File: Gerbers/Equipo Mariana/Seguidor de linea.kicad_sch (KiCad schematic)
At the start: 23 parts, among them J1 VCC, J11 I2C PROTOCOL, J2 MOTOR A, J3 MOTOR B, J4 Regleta_Jabots, J5 TURBIBNA, J7 Conn_02x01, SW1 SW_SPDT, U2 ESP32-DEVKIT-V1, U3 LM7805, U4 ROB-14450

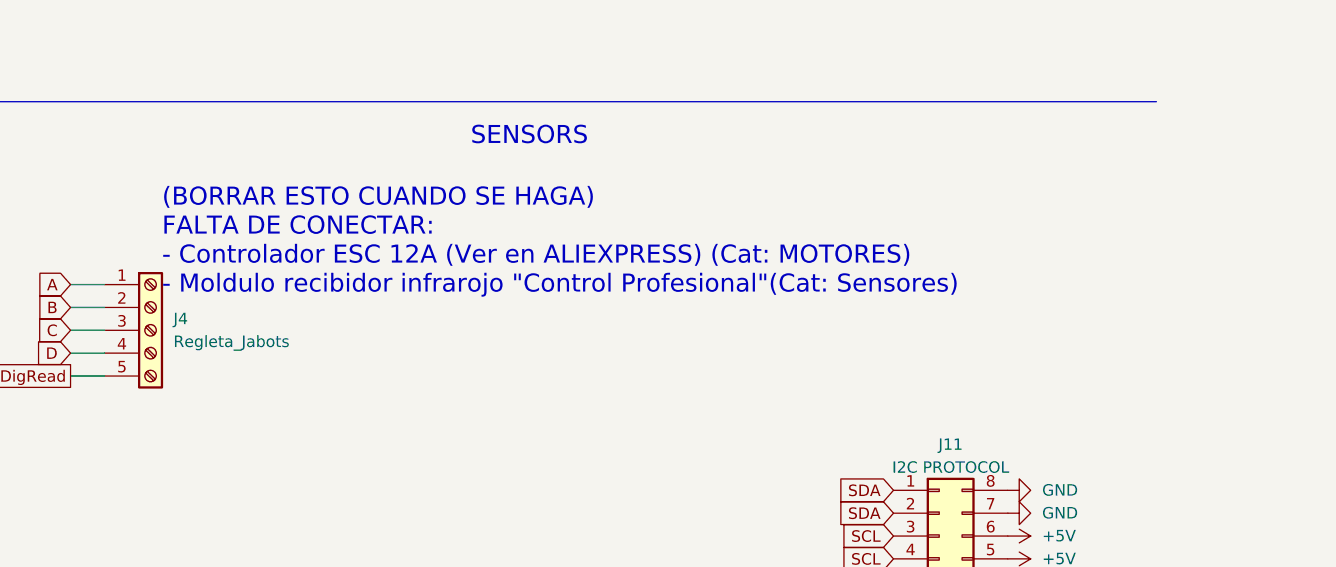
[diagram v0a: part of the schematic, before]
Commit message: Puse un punto
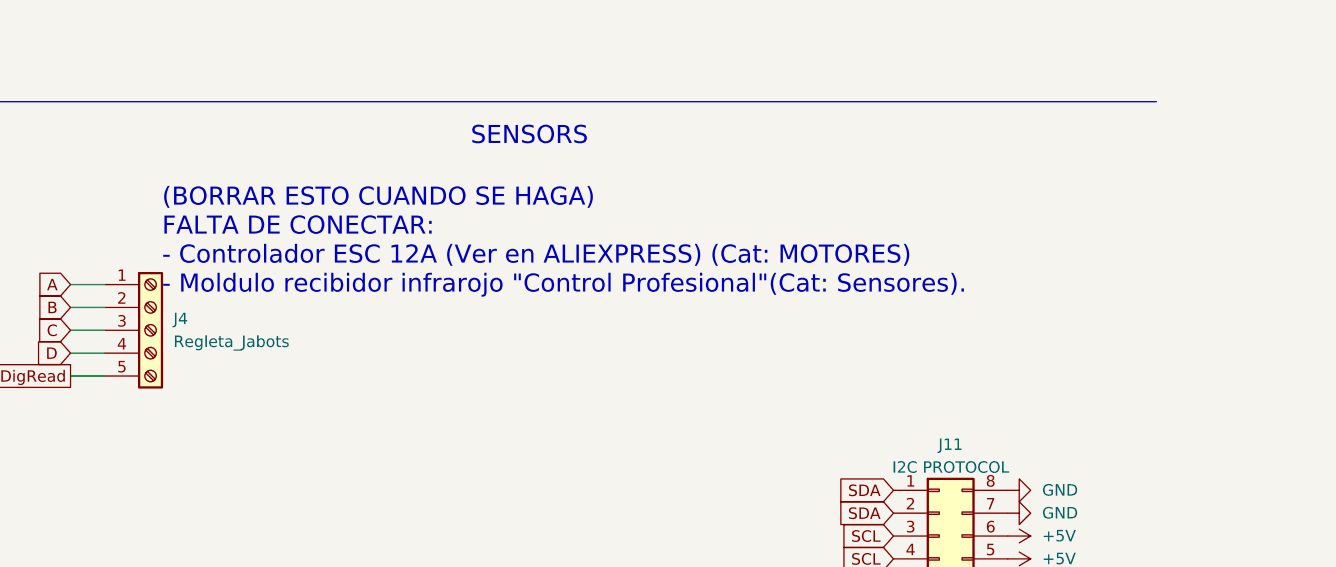
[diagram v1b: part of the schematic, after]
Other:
- note added: "(BORRAR ESTO CUANDO SE HAGA) FALTA DE CONECTAR: - Controlador ESC 12A (Ver en ALIEXPRESS) (Cat: MOTORES) - Moldulo recibidor infrarojo "Control Profesional"(Cat: Sensores)."
- note removed: "(BORRAR ESTO CUANDO SE HAGA) FALTA DE CONECTAR: - Controlador ESC 12A (Ver en ALIEXPRESS) (Cat: MOTORES) - Moldulo recibidor infrarojo "Control Profesional"(Cat: Sensores)"
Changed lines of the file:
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@@
     (effects (font (size 6 6) (color 0 0 0 1)) (justify left bottom))
   )
-  (text "(BORRAR ESTO CUANDO SE HAGA)\nFALTA DE CONECTAR:\n- Controlador ESC 12A (Ver en ALIEXPRESS) (Cat: MOTORES)\n- Moldulo recibidor infrarojo \"Control Profesional\"(Cat: Sensores)"
+  (text "(BORRAR ESTO CUANDO SE HAGA)\nFALTA DE CONECTAR:\n- Controlador ESC 12A (Ver en ALIEXPRESS) (Cat: MOTORES)\n- Moldulo recibidor infrarojo \"Control Profesional\"(Cat: Sensores)."
     (at 173.99 92.71 0)
     (effects (font (size 2 2) (color 0 0 0 1)) (justify left bottom))
